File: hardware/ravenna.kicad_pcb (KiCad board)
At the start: 4 copper layers, 22.9 x 71.9 mm, 68 parts, among them IC2 FT232H, IC3 MCP1755, IC4 93C56, IC5 RAVENAQFN56, J7 47491-0001, J9 2X6 FEMALE, U2 W25Q32FV, X1 12MHZ, X2 8MHZ

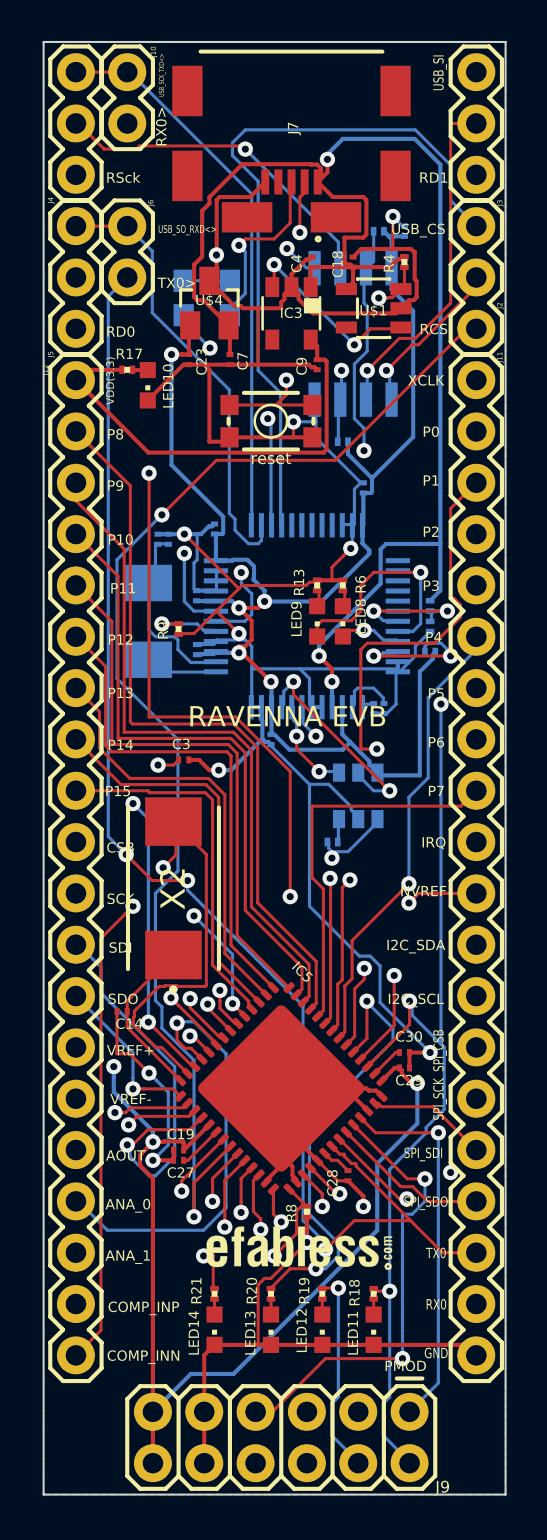
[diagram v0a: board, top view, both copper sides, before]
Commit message: parts libraries
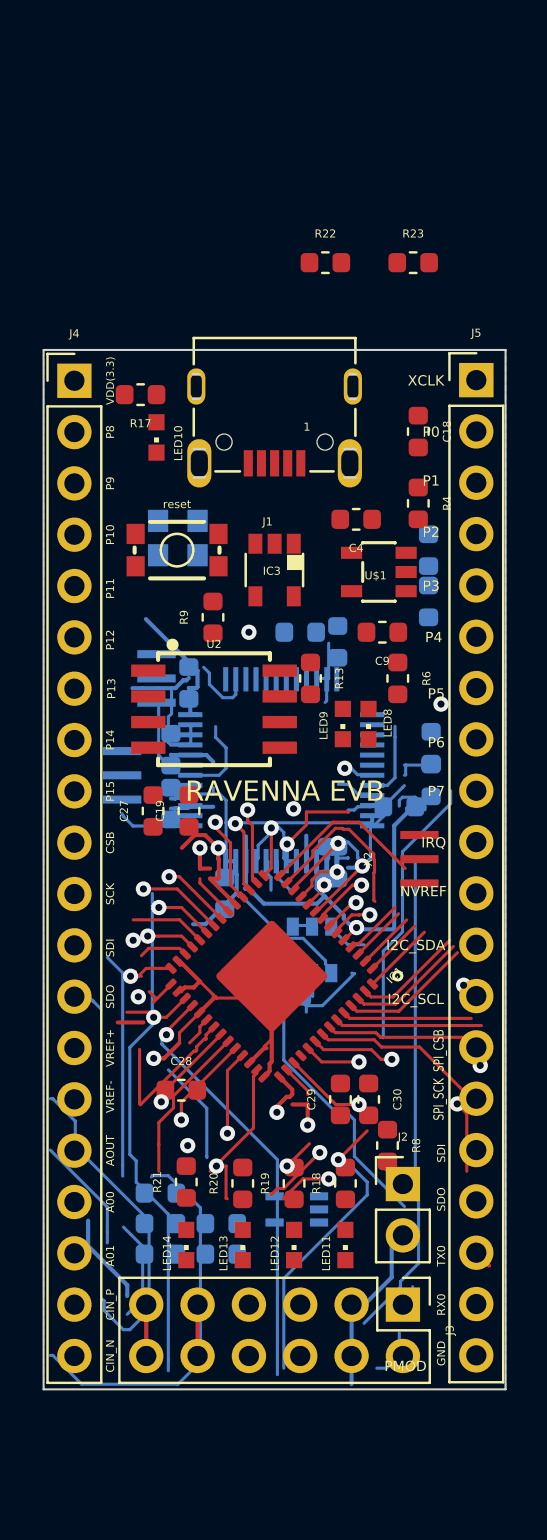
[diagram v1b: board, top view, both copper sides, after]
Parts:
- removed C1, C14, C2, C3: 27pf, C0201
- removed C23: 2.2uf, C0201
- removed C7: 1uf, C0201
- removed G***: LOGO, raptor-KiCadVersion:logo
- removed IC5: RAVENAQFN56, QFN56
- removed J10, J6: , 1X02
- removed J11, J12: , 1X20
- removed J7: 47491-0001, 47491-0001
- removed J9: 2X6 FEMALE, 2X6
- removed RESET: SPST-SMD-4.6X2.8mm, TACTILE_SWITCH_SMD_4.6X2.8MM
- removed U$4: MCP1811, SOT23
- added IC1: RAVENAQFN56, parts and footprints:QFN56, F.Cu at (148.3, 115.2)
- added J1: 629105150521, parts and footprints:629105150521, F.Cu at (148.5, 88.8)
- added R10: 10K, parts and footprints:R_0603_1608Metric, B.Cu at (142.8, 127.4)
- added R11: 10K, parts and footprints:R_0603_1608Metric, B.Cu at (145.8, 128.9)
- added R15: 10K, parts and footprints:R_0603_1608Metric, B.Cu at (142.8, 125.9)
- added R16: 10K, parts and footprints:R_0603_1608Metric, B.Cu at (145.8, 127.4)
- added R22: 0, Resistor_SMD:R_0603_1608Metric, F.Cu at (151.0, 79.9)
- added R23: 10K, Resistor_SMD:R_0603_1608Metric, F.Cu at (155.3, 79.9)
- added R3: 10K, parts and footprints:R_0603_1608Metric, B.Cu at (142.8, 128.9)
- added REF**: CSTNE12M0GH5L000R0, parts and footprints:CSTNE12M0GH5L000R0, B.Cu at (142.6, 100.5)
- added RESET1: SPST-SMD-4.6X2.8mm, parts and footprints:TACTILE_SWITCH_SMD_4.6X2.8MM, F.Cu at (143.6, 94.1)
- added U1: SN74LVC1G125DCKR, parts and footprints:SC-70-5, B.Cu at (149.6, 126.7)
- C15, C16, C17, C18, C19, C20, C21, C22, C27, C28, C29, C30, C4, C5, C8, C9: footprint C0201 -> Capacitor_SMD:C_0603_1608Metric
- J2: value (none) -> Conn_01x02_Male; footprint 1X03 -> Connector_PinHeader_2.54mm:PinHeader_1x02_P2.54mm_Vertical
- J3: value (none) -> 2X6 FEMALE; footprint 1X03 -> Connector_PinHeader_2.54mm:PinHeader_2x06_P2.54mm_Vertical
- J4, J5: value (none) -> CONN_20; footprint 1X03 -> Connector_PinHeader_2.54mm:PinHeader_1x20_P2.54mm_Vertical
- LED10, LED11, LED12, LED13, LED14, LED8, LED9: value (none) -> LEDCHIPLED_0603
- R1, R12, R13, R17, R18, R19, R20, R21, R4, R5, R6, R7, R8: footprint R0201 -> Resistor_SMD:R_0603_1608Metric
- R14, R2: value 4.7K -> 10K; footprint R0201 -> Resistor_SMD:R_0603_1608Metric
- R9: value 2K 1% -> 12K 1%; footprint R0201 -> Resistor_SMD:R_0603_1608Metric
- U2: moved to F.Cu
- X1: value 12MHZ -> 12MHz; footprint 445I23D24M00000 -> parts and footprints:CSTNE12M0GH5L000R0
- X2: value 8MHZ -> 6 MHz; footprint CX8045GA04000H0PST03 -> CSTNE12M0GH5L000R0
- moved J3 56.0 mm to (154.8, 131.4), turned to 270 degrees
- moved J2 42.5 mm to (154.8, 125.5), turned to 0 degrees
- moved J5 20.0 mm to (158.4, 85.7), turned to 0 degrees
- moved U2 19.8 mm to (145.5, 102.0), turned to 270 degrees
- moved R12 18.5 mm to (156.1, 96.6), turned to 90 degrees
- moved C27 17.3 mm to (142.5, 107.0), turned to 90 degrees
- moved C19 16.8 mm to (144.2, 107.0), turned to 90 degrees
- moved C5 15.8 mm to (156.1, 94.1)
- moved C9 13.6 mm to (153.8, 98.2), turned to 180 degrees
- moved U$1 13.1 mm to (153.6, 95.2)
- moved C4 12.9 mm to (152.5, 92.6), turned to 180 degrees
- moved IC3 12.7 mm to (148.5, 95.1)
- moved X2 12.3 mm to (155.6, 109.4)
- moved FUSE_0 12.0 mm to (144.7, 93.5)
- moved R4 12.0 mm to (155.6, 91.8), turned to 270 degrees
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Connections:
- C15 pad 2: +3V3 -> +5V
- C16 pad 1: +3V3 -> +5V
- C17 pad 1: +3V3 -> +5V
- C19 pad 1: VDD(3.3) -> +5V
- C20 pad 1: +3V3 -> +5V
- C21 pad 1: +3V3 -> +5V
- C29 pad 2: VDD(3.3) -> +5V
- C5 pad 2: +3V3 -> +5V
- C9 pad 1: VDD(3.3) -> +5V
- IC2 pad 12: +3V3 -> +5V
- IC2 pad 13: USB_SCK_TXD -> /TXD_HK_SCK
- IC2 pad 14: USB_SO_RXD -> /RXD_HK_SDI
- IC2 pad 15: USB_SI -> /HK_SDO
- IC2 pad 16: USB_CS -> /HK_CSB
- IC2 pad 17: (no net) -> Net-(IC2-Pad17)
- IC2 pad 18: (no net) -> Net-(IC2-Pad18)
- IC2 pad 19: (no net) -> Net-(IC2-Pad19)
- IC2 pad 2: N$11 -> Net-(IC2-Pad2)
- IC2 pad 20: (no net) -> Net-(IC2-Pad20)
- IC2 pad 21: (no net) -> /TMUX_SEL
- IC2 pad 24: +3V3 -> +5V
- IC2 pad 25: (no net) -> /TXD_EN
- IC2 pad 26: (no net) -> Net-(IC2-Pad26)
- IC2 pad 27: (no net) -> Net-(IC2-Pad27)
- IC2 pad 28: (no net) -> Net-(IC2-Pad28)
- IC2 pad 29: (no net) -> Net-(IC2-Pad29)
- IC2 pad 3: +3V3 -> +5V
- IC2 pad 30: (no net) -> Net-(IC2-Pad30)
- IC2 pad 31: N$27 -> Net-(IC2-Pad31)
- IC2 pad 39: +3V3 -> +5V
- IC2 pad 44: N$8 -> Net-(IC2-Pad44)
- IC2 pad 46: +3V3 -> +5V
- IC2 pad 8: +3V3 -> +5V
- IC3 pad 4: (no net) -> Net-(IC3-Pad4)
- IC3 pad 5: VDD(3.3) -> +5V
- IC4 pad 4: N$8 -> Net-(IC2-Pad44)
- IC4 pad 6: +3V3 -> +5V
- J2 pad 1: RAPTOR_CS -> GND
- J2 pad 2: N$14 -> /TXD_EN
- J3 pad 1: RAPTOR_D1 -> /SPI_CSB
- J3 pad 2: N$15 -> /P0
- J3 pad 3: USB_SI -> /SPI_SDO
- J4 pad 1: RAPTOR_SCK -> +5V
- J4 pad 2: N$17 -> /P8
- J4 pad 3: USB_SCK_TXD -> /P9
- J5 pad 1: RAPTOR_D0 -> /XCLK
- J5 pad 2: N$16 -> /P0
- J5 pad 3: USB_SO_RXD -> /P1
- R1 pad 1: RAPTOR_D2 -> +5V
- R1 pad 2: +3V3 -> /RAPTOR_D2
- R12 pad 1: RAPTOR_D3 -> +5V
- R12 pad 2: +3V3 -> /RAPTOR_D3
- R13 pad 1: GND -> +5V
- R14 pad 1: N$27 -> +5V
- R14 pad 2: +5V -> Net-(IC2-Pad44)
- R17 pad 2: VDD(3.3) -> +5V
- R18 pad 2: P0 -> /P0
- R19 pad 2: P1 -> /P1
- R2 pad 1: GND -> +5V
- R2 pad 2: N$27 -> /RAPTOR_CS
- R20 pad 2: P2 -> /P2
- R21 pad 2: P3 -> /P3
- R5 pad 2: +3V3 -> +5V
- R6 pad 1: GND -> +5V
- R8 pad 1: IRQ -> /IRQ
- U$1 pad 5: (no net) -> Net-(U$1-Pad5)
- U2 pad 1: N$14 -> /RAPTOR_CS
- U2 pad 2: N$15 -> /RAPTOR_D1
- U2 pad 3: RAPTOR_D2 -> /RAPTOR_D2
- U2 pad 5: N$16 -> /RAPTOR_D0
- U2 pad 6: N$17 -> /RAPTOR_SCK
- U2 pad 7: RAPTOR_D3 -> /RAPTOR_D3
- U2 pad 8: +3V3 -> +5V
- X1 pad 2: N$11 -> GND
- X2 pad 2: N$10 -> GND
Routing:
- net GND: track 226.6 -> 116.2 mm, vias 12 -> 3
- net VDD(3.3): track 109.2 -> 0.00 mm, vias 3 -> 0
- net /P2: track 0.00 -> 99.8 mm, vias 0 -> 1
- net +3V3: track 77.3 -> 0.00 mm, vias 5 -> 0
- net RX0: track 75.1 -> 0.00 mm, vias 3 -> 0
- net RAPTOR_D1: track 73.9 -> 0.00 mm, vias 1 -> 0
- net TX0: track 68.2 -> 0.00 mm, vias 3 -> 0
- net /XCLK: track 0.00 -> 64.0 mm, vias 0 -> 1
- net RAPTOR_SCK: track 62.8 -> 0.00 mm, vias 1 -> 0
- net P1: track 61.9 -> 0.00 mm, vias 3 -> 0
- net RAPTOR_CS: track 61.8 -> 0.00 mm, vias 2 -> 0
- net P0: track 61.7 -> 0.00 mm, vias 3 -> 0
- net (no net): track 0.00 -> 61.0 mm, vias 0 -> 3
- net /SPI_CSB: track 0.00 -> 60.5 mm, vias 0 -> 2
- net RAPTOR_D3: track 55.7 -> 0.00 mm, vias 2 -> 0
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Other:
- board size 22.9 x 71.9 mm -> 22.9 x 51.4 mm
- board text added: "A00"
- board text added: "A01"
- board text added: "CIN_N"
- board text added: "CIN_P"
- board text removed: "ANA_0"
- board text removed: "ANA_1"
- board text removed: "COMP_INN"
- board text removed: "COMP_INP"
- board text removed: "RCS"
- board text removed: "RD0"
- board text removed: "RD1"
- board text removed: "RSck"
- board text removed: "RX0>"
- board text removed: "SPI_SDI"
- board text removed: "SPI_SDO"
- board text removed: "TX0>"
- board text removed: "USB_CS"
- board text removed: "USB_SCK_TXD<>"
- board text removed: "USB_SI"
- board text removed: "USB_SO_RXD<>"
